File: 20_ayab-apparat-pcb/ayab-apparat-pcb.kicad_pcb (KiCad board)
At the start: 2 copper layers, 58 parts, among them K1 CONN_3, K2 CONN_3, P1 CONN_4, P10 CONN_2, P2 CONN_10, P3 CONN_10, P4 CONN_8, P5 CONN_5, P6 CONN_5, P7 CONN_3X2, P8 CONN_4, P9 CONN_2, Q1 MOSFET_P, SW1 SW_PUSH, U1 LM1117, U2 PCF8574, U3 PCF8574, U4 ULN2803, U5 ULN2803, U6 ATMEGA32U4-A, X1 16MHz, X2 USBMINI

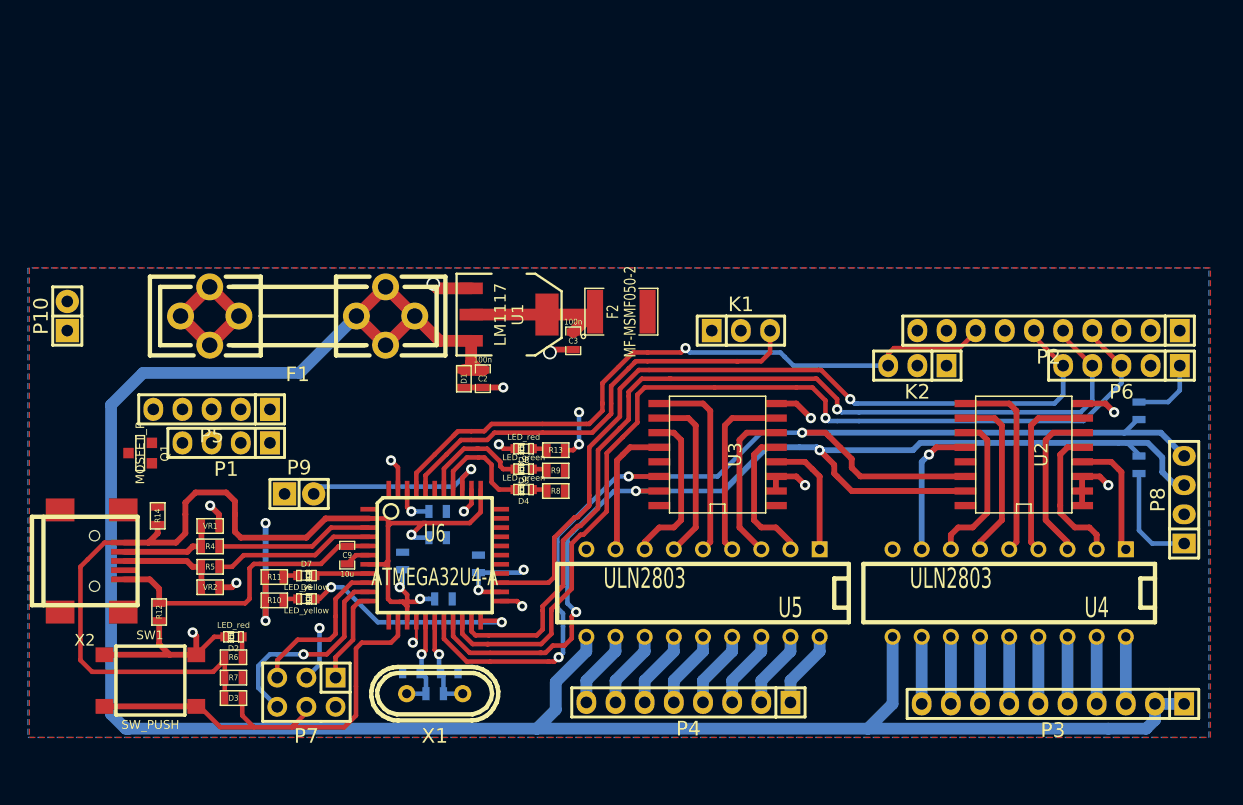
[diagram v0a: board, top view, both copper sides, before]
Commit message: PCB Version for final Review
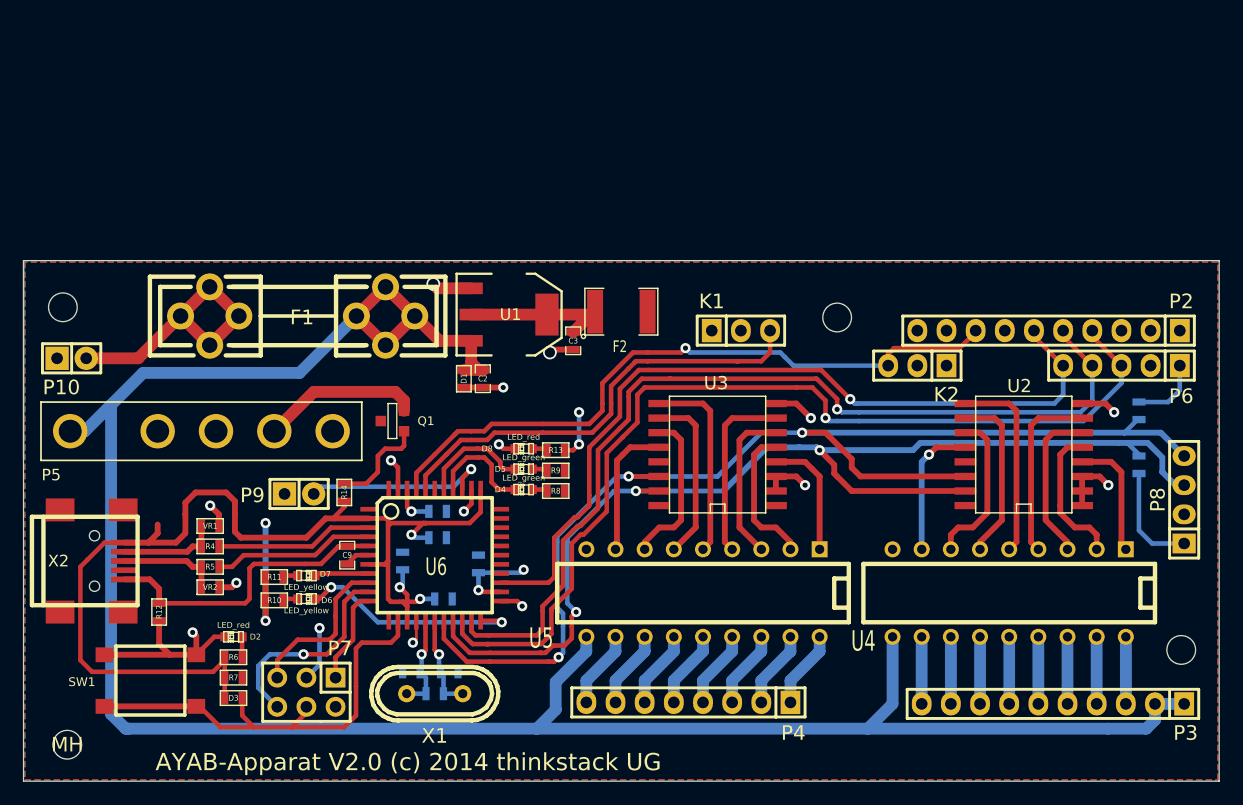
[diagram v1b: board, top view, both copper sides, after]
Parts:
- removed P1: CONN_4, Pin_Headers:Pin_Header_Straight_1x04
- added ASTUB: VAL**, ASTUB, F.Cu at (110.7, 63.1)
- added MH: MountingHole_2-5mm_RevA_Date21Jun2010, Mounting_Holes:MountingHole_2-5mm, F.Cu at (63.5, 126.0)
- added MH: MountingHole_2-5mm_RevA_Date21Jun2010, Mounting_Holes:MountingHole_2-5mm, F.Cu at (160.5, 117.7)
- added MH: MountingHole_2-5mm_RevA_Date21Jun2010, Mounting_Holes:MountingHole_2-5mm, F.Cu at (63.1, 87.9)
- added MH: MountingHole_2-5mm_RevA_Date21Jun2010, Mounting_Holes:MountingHole_2-5mm, F.Cu at (130.6, 88.8)
- P5: footprint Pin_Headers:Pin_Header_Straight_1x05 -> ayab:KH-930_PWR_CON
- moved Q1 22.1 mm to (91.8, 97.8)
- moved R14 16.4 mm to (87.6, 104.0)
- moved P5 12.5 mm to (63.8, 98.7), turned to 0 degrees
- moved P10 3.70 mm to (63.9, 92.3), turned to 0 degrees
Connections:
- U1 pad 4: Net-(C3-Pad1) -> (no net)
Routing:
- net +5V_MACHINE: track 0.00 -> 13.9 mm
- net Net-(F1-Pad2): track 14.4 -> 24.1 mm
- net Net-(Q1-PadG): track 0.00 -> 8.66 mm
- net +12V: track 191.0 -> 195.5 mm
- net VUSB: track 94.4 -> 96.4 mm
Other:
- board outline added: 104.1 x 45.3 mm
- board text added: "AYAB-Apparat V2.0 (c) 2014 thinkstack UG"
